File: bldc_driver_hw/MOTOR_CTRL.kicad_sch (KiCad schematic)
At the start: 0 parts

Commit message: wip
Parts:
- added C17: C_Snub, Capacitor_SMD:C_0805_2012Metric_Pad1.18x1.45mm_HandSolder, symbol Device:C_Small
- added C18: C_Small, Capacitor_SMD:C_0805_2012Metric_Pad1.18x1.45mm_HandSolder, symbol Device:C_Small
- added D2, D3, D5, D6: D_Schottky, symbol Device:D_Schottky
- added IC1: DRV8334PHPR, QFP50P900X900X120-49N, symbol bldc_driver_lib:DRV8334PHPR
- added Q1, Q2: NMOS, symbol Simulation_SPICE:NMOS
- added R11, R12, R14, R9: R_GATE, symbol Device:R_Small
- added R13, R15: R_GS, symbol Device:R_Small
- added R4: SHUNT, symbol Device:R_Small
- added R7: R_snub, symbol Device:R_Small
- added R8: C_snub, symbol Device:R_Small
- added TP2, TP3: TestPoint, symbol Connector:TestPoint
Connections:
- new net: D6.1 (K), R9.1
- new net: Q2.2 (G), R13.2, R14.2, R9.2, TP3.1
- new net: D6.2 (A), R14.1
- new net: C17.2, R7.1
- new net: Q1.2 (G), R11.2, R12.2, R15.2, TP2.1
- new net: D2.2 (A), Q2.3 (S), R13.1, R4.1
- new net: D5.1 (K), R11.1
- new net: D5.2 (A), R12.1
- new net: C18.2, R8.1
- new net +48V: D3.1 (K), Q1.1 (D), R8.2
- new net GND: R4.2, R7.2
- new net PHASE_A: C17.1, C18.1, D2.1 (K), D3.2 (A), Q1.3 (S), Q2.1 (D), R15.1

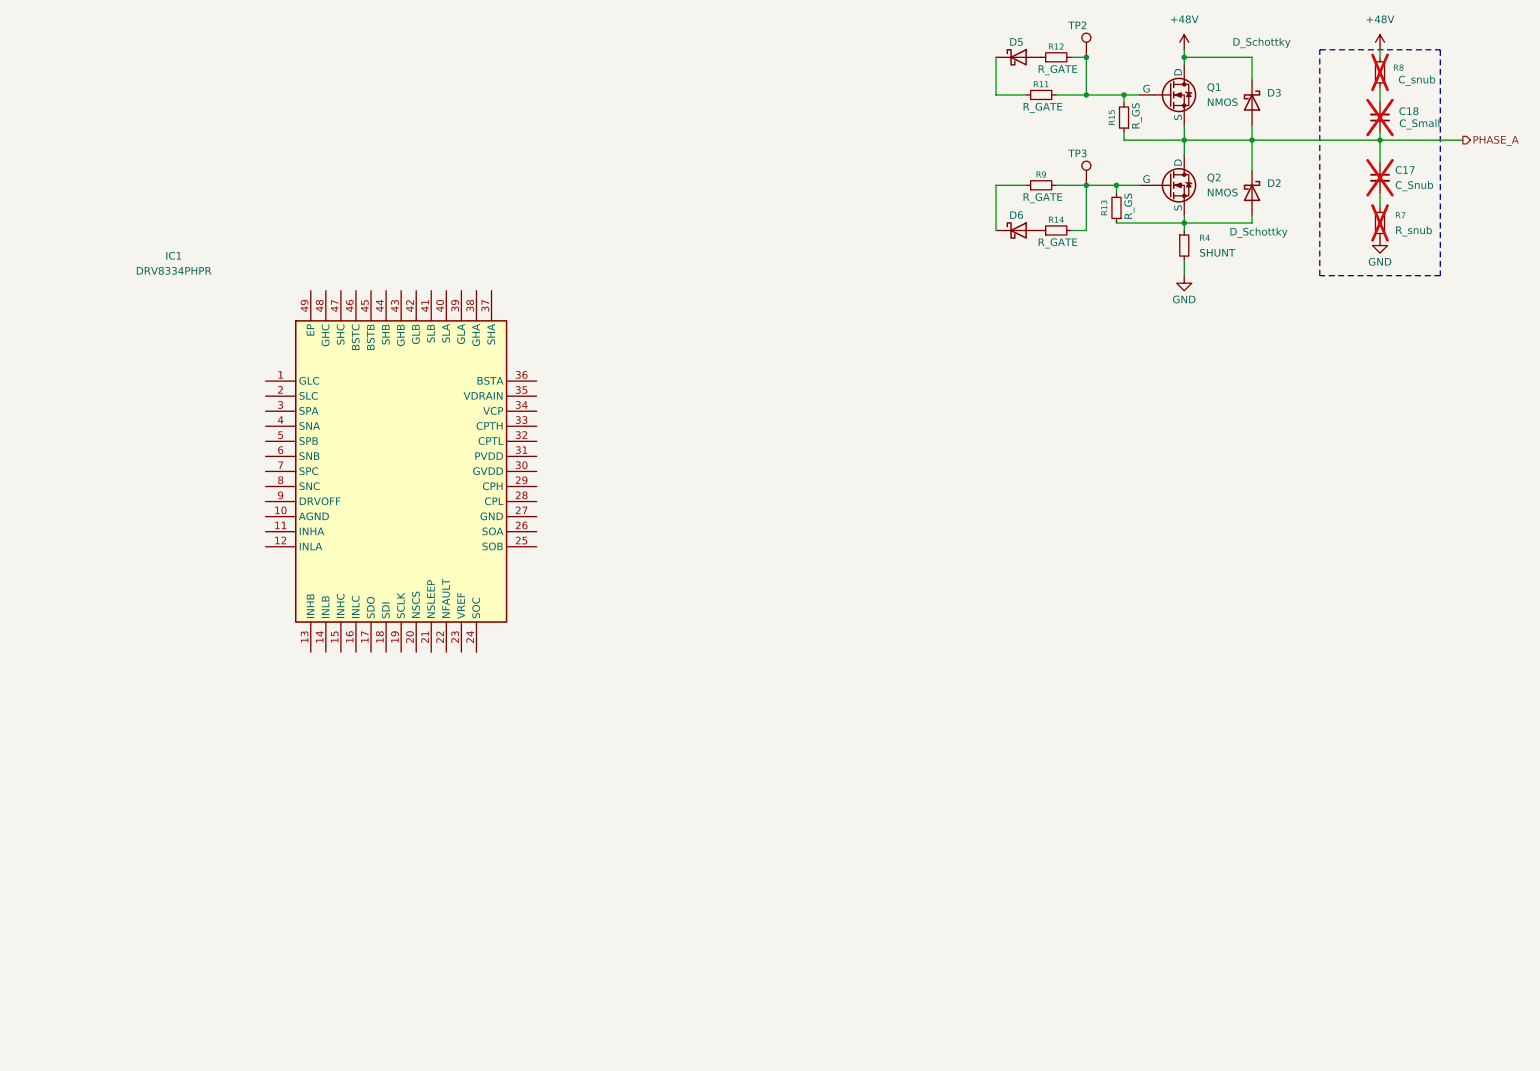
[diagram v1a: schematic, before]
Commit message: wip
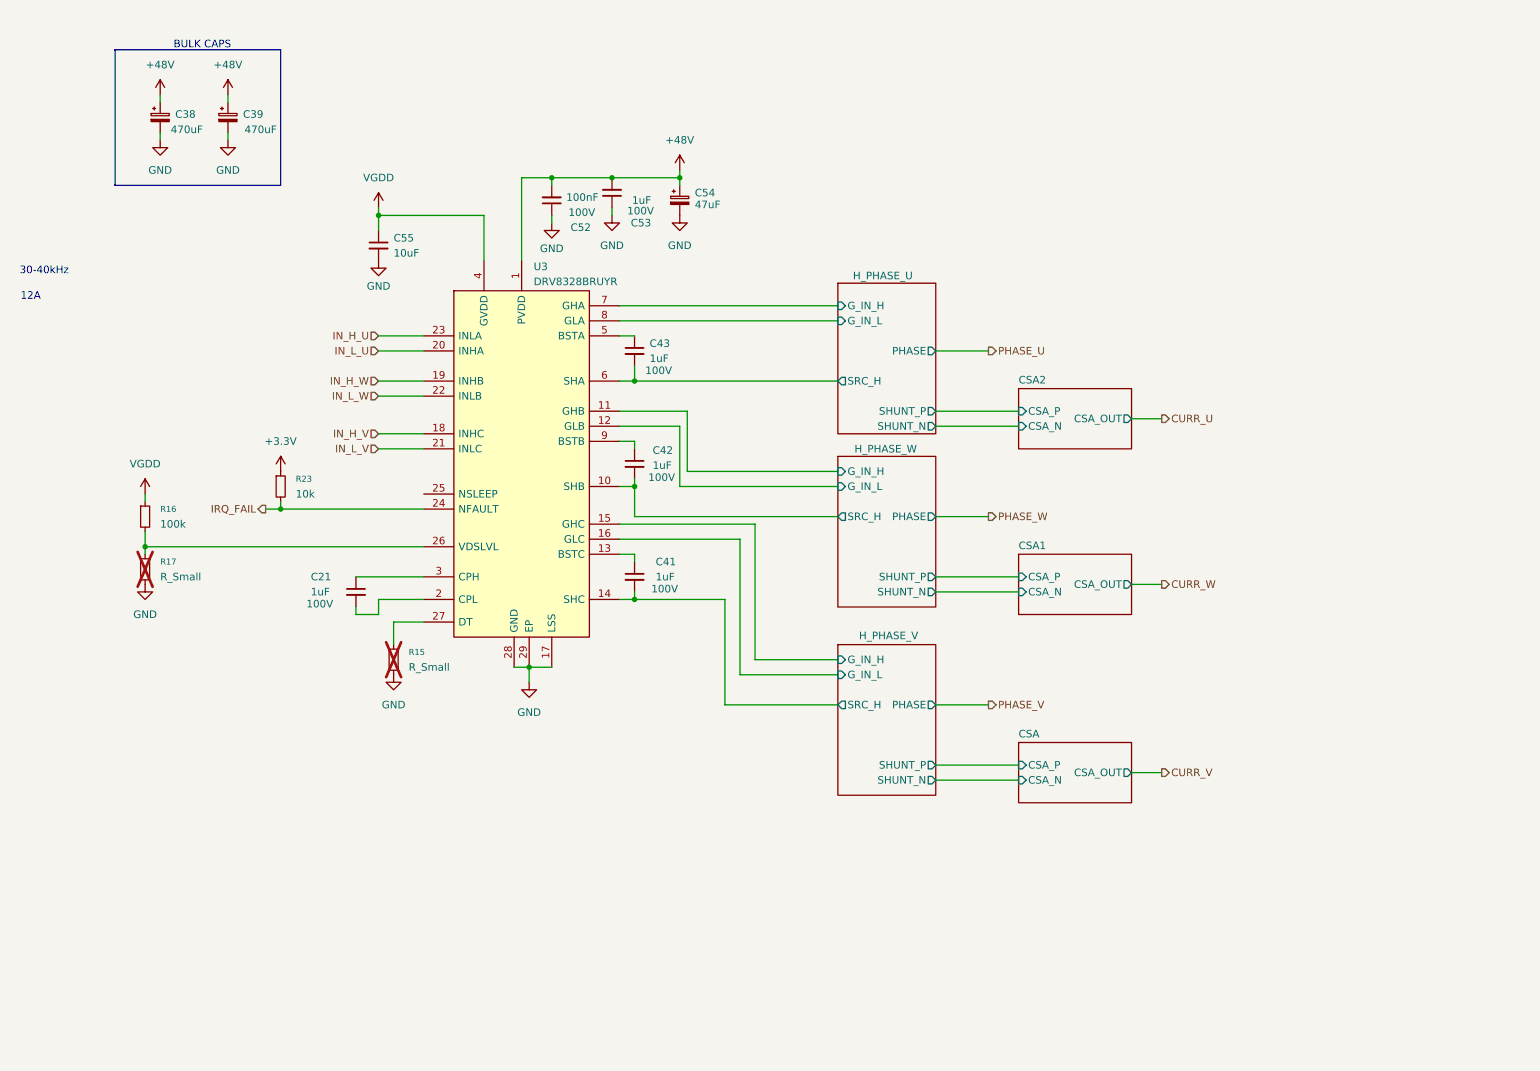
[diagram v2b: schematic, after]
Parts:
- removed C17: C_Snub, Capacitor_SMD:C_0805_2012Metric_Pad1.18x1.45mm_HandSolder, symbol Device:C_Small
- removed C18: C_Small, Capacitor_SMD:C_0805_2012Metric_Pad1.18x1.45mm_HandSolder, symbol Device:C_Small
- removed D2, D3, D5, D6: D_Schottky, symbol Device:D_Schottky
- removed IC1: DRV8334PHPR, QFP50P900X900X120-49N, symbol bldc_driver_lib:DRV8334PHPR
- removed Q1, Q2: NMOS, symbol Simulation_SPICE:NMOS
- removed R11, R12, R14, R9: R_GATE, symbol Device:R_Small
- removed R13: R_GS, symbol Device:R_Small
- removed R4: SHUNT, symbol Device:R_Small
- removed R7: R_snub, symbol Device:R_Small
- removed R8: C_snub, symbol Device:R_Small
- removed TP2, TP3: TestPoint, symbol Connector:TestPoint
- added C21, C41, C42, C43, C53: 1uF, Capacitor_SMD:C_0805_2012Metric, symbol Device:C_Small
- added C38, C39: 470uF, symbol Device:C_Polarized_Small
- added C52: 100nF, Capacitor_SMD:C_0805_2012Metric, symbol Device:C_Small
- added C54: 47uF, symbol Device:C_Polarized_Small
- added C55: 10uF, Capacitor_SMD:C_0805_2012Metric, symbol Device:C_Small
- added R16: 100k, symbol Device:R_Small
- added R17: R_Small, symbol Device:R_Small
- added R23: 10k, symbol Device:R_Small
- added U3: DRV8328BRUYR, bldc_driver_footprint:QFN40P400X400X80-29N-D, symbol bldc_driver_lib:DRV8328BRUYR
- R15: value R_GS -> R_Small; now not fitted
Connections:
- net +48V: now also C38.1, C39.1, C52.2, C53.2, C54.1, U3.1 (PVDD)
- net GND: now also R15.2, C38.2, C39.2, C52.1, C53.1, C54.2, C55.2, R17.2, U3.17 (LSS), U3.28 (GND), U3.29 (EP)
- net PHASE_A: no longer names the net of R15.1
- net PHASE_A: now also U3.27 (DT)
- new net: R16.2, R17.1, U3.26 (VDSLVL)
- new net: C21.1, U3.3 (CPH)
- new net: C21.2, U3.2 (CPL)
- new net: C42.1, U3.9 (BSTB)
- new net: C41.1, U3.13 (BSTC)
- new net: C43.1, U3.5 (BSTA)
- new net +3.3V: R23.1
- new net H_PHASE_U/G_IN_H: U3.7 (GHA)
- new net H_PHASE_U/G_IN_L: U3.8 (GLA)
- new net H_PHASE_U/SRC_H: C43.2, U3.6 (SHA)
- new net H_PHASE_V/G_IN_H: U3.15 (GHC)
- new net H_PHASE_V/G_IN_L: U3.16 (GLC)
- new net H_PHASE_V/SRC_H: C41.2, U3.14 (SHC)
- new net H_PHASE_W/G_IN_H: U3.11 (GHB)
- new net H_PHASE_W/G_IN_L: U3.12 (GLB)
- new net H_PHASE_W/SRC_H: C42.2, U3.10 (SHB)
- new net IN_H_U: U3.23 (INLA)
- new net IN_H_V: U3.18 (INHC)
- new net IN_H_W: U3.19 (INHB)
- new net IN_L_U: U3.20 (INHA)
- new net IN_L_V: U3.21 (INLC)
- new net IN_L_W: U3.22 (INLB)
- new net IRQ_FAIL: R23.2, U3.24 (NFAULT)
- new net VGDD: C55.1, R16.1, U3.4 (GVDD)
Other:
- added sheet CSA (CSA.kicad_sch)
- added sheet CSA1 (CSA.kicad_sch)
- added sheet CSA2 (CSA.kicad_sch)
- added sheet H_PHASE_U (H_BRIDGE.kicad_sch)
- added sheet H_PHASE_V (H_BRIDGE.kicad_sch)
- added sheet H_PHASE_W (H_BRIDGE.kicad_sch)
- note added: "12A"
- note added: "30-40kHz"
- note added: "BULK CAPS"

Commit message: wip
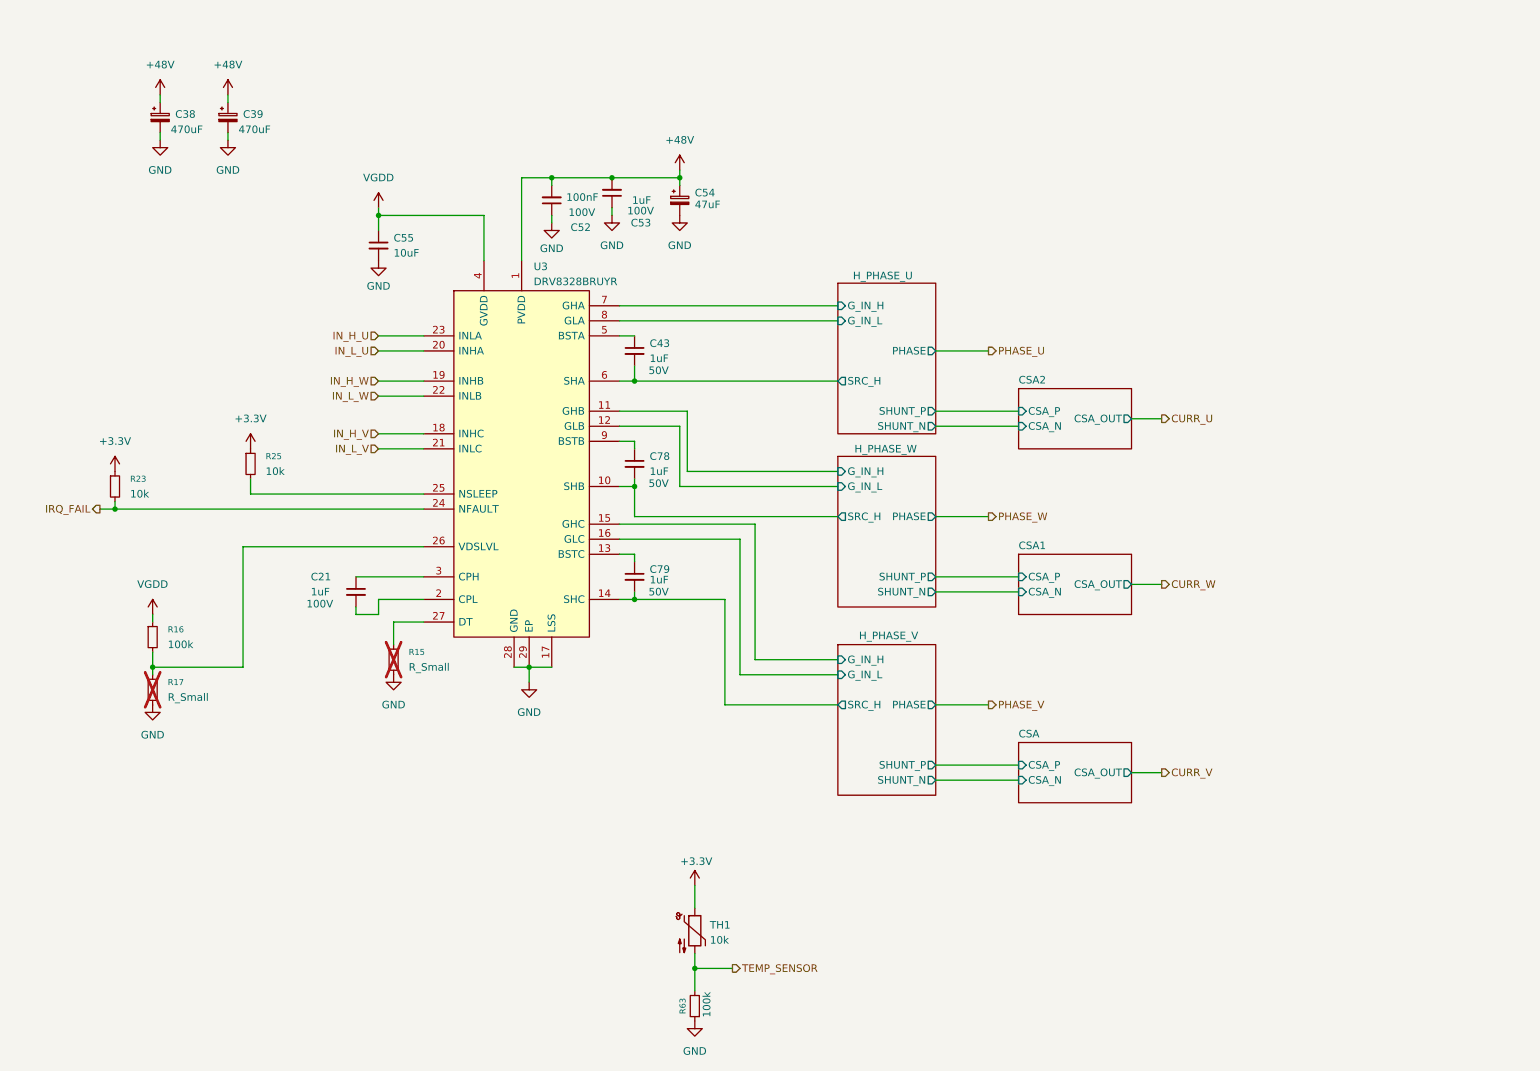
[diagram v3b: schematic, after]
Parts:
- removed C41, C42: 1uF, Capacitor_SMD:C_0805_2012Metric, symbol Device:C_Small
- added C78, C79: 1uF, Capacitor_SMD:C_0603_1608Metric_Pad1.08x0.95mm_HandSolder, symbol Device:C_Small
- added R25: 10k, Resistor_SMD:R_0603_1608Metric, symbol Device:R_Small
- added R63: 100k, Resistor_SMD:R_0805_2012Metric, symbol Device:R_Small
- added TH1: 10k, Resistor_SMD:R_0603_1608Metric, symbol Device:Thermistor_NTC
- C38, C39: footprint (none) -> Capacitor_THT:CP_Radial_D16.0mm_P7.50mm
- C43: footprint Capacitor_SMD:C_0805_2012Metric -> Capacitor_SMD:C_0603_1608Metric_Pad1.08x0.95mm_HandSolder; Rating 100V -> 50V
- C54: footprint (none) -> Capacitor_THT:CP_Radial_D10.0mm_P5.00mm
- C55: footprint Capacitor_SMD:C_0805_2012Metric -> Capacitor_SMD:C_0603_1608Metric
- R15, R16, R17, R23: footprint (none) -> Resistor_SMD:R_0603_1608Metric
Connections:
- net +3.3V: now also R25.1, TH1.1
- net GND: now also R63.1
- net H_PHASE_V/SRC_H: now also C79.2
- net H_PHASE_W/SRC_H: now also C78.2
- net at U3.9 (BSTB): now also C78.1
- net at U3.13 (BSTC): now also C79.1
- net at U3.25 (NSLEEP): now also R25.2
- new net TEMP_SENSOR: R63.2, TH1.2
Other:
- note removed: "12A"
- note removed: "30-40kHz"
- note removed: "BULK CAPS"
- moved on the sheet: R16, R17, R23
